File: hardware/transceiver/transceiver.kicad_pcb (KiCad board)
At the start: 4 copper layers, 30 x 30 mm, 49 parts, among them J1 Conn_01x04, J2 Conn_01x02, J3 Conn_Coaxial, U1 SX1262IMLTRT, U2 AP2112K-3.3, U3 PE4259, U4 STM32U585CIUx, Y1 32MHz, Y2 Q13FC13500004, Y3 X322516MLB4SI

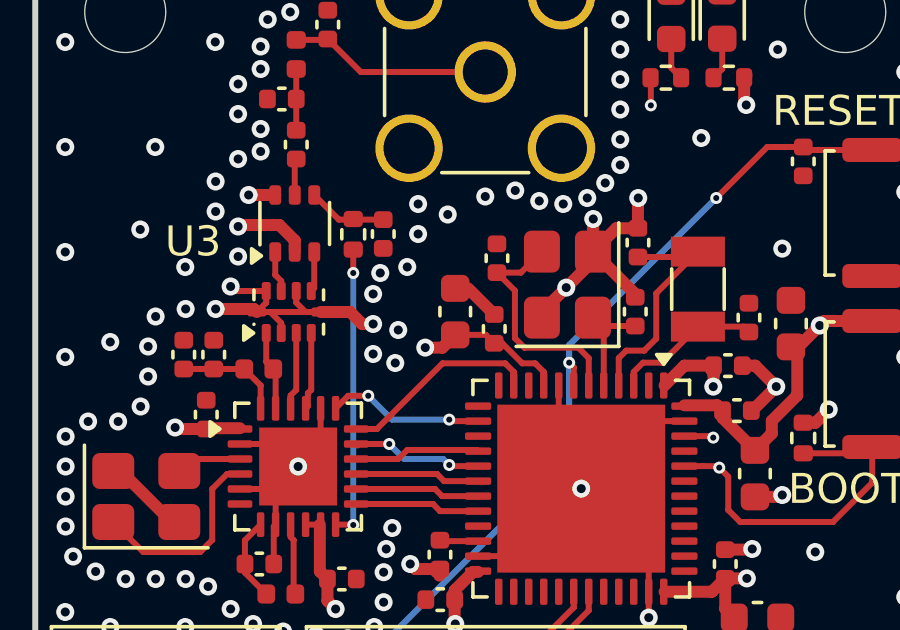
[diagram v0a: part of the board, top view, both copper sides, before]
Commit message: updated cad
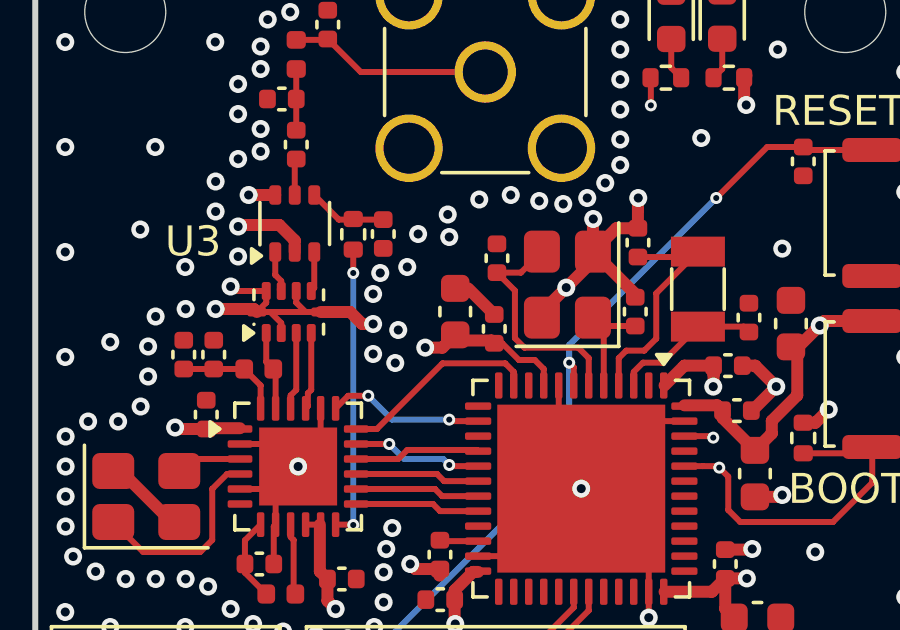
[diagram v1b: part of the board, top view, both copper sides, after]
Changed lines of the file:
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@@
 	)
 	(via
-		(at 141 102.95)
+		(at 140.85 103.1)
 		(size 0.6)
 		(drill 0.3)
@@
 	)
 	(via
-		(at 140 103.15)
+		(at 139.8 103.25)
 		(size 0.6)
 		(drill 0.3)
@@
 	)
 	(via
-		(at 137.7625 103.4)
+		(at 138.8 104.5)
 		(size 0.6)
 		(drill 0.3)
@@
 	)
 	(segment
-		(start 140.02 107.7625)
-		(end 140.3 108.0425)
+		(start 141.123703 108.6)
+		(end 141.65 108.6)
 		(width 0.2)
 		(layer "F.Cu")
@@
 	)
 	(segment
-		(start 141.664799 108.7115)
-		(end 141.95 108.996701)
-		(width 0.2)
-		(layer "F.Cu")
-		(net 3)
-	)
-	(segment
 		(start 148 115.88)
 		(end 147.555 116.325)
@@
 	)
 	(segment
-		(start 141.235203 108.7115)
-		(end 141.664799 108.7115)
+		(start 141.65 108.6)
+		(end 141.95 108.9)
+		(width 0.2)
+		(layer "F.Cu")
+		(net 3)
+	)
+	(segment
+		(start 140.3 108.0425)
+		(end 140.566203 108.0425)
 		(width 0.2)
 		(layer "F.Cu")
@@
 	)
 	(segment
-		(start 141.95 108.996701)
-		(end 141.95 109.45)
-		(width 0.2)
-		(layer "F.Cu")
-		(net 3)
-	)
-	(segment
 		(start 129.7125 110.9)
 		(end 130.7 110.9)
@@
 	)
 	(segment
-		(start 140.566203 108.0425)
-		(end 141.235203 108.7115)
-		(width 0.2)
+		(start 140.2075 107.95)
+		(end 140.3 108.0425)
+		(width 0.4)
 		(layer "F.Cu")
 		(net 3)
@@
 	)
 	(segment
-		(start 139 107.7625)
-		(end 140.02 107.7625)
-		(width 0.2)
-		(layer "F.Cu")
-		(net 3)
-	)
-	(segment
 		(start 147.555 116.325)
 		(end 145.976 116.325)
@@
 	)
 	(segment
-		(start 139.28 108.0425)
-		(end 139 107.7625)
-		(width 0.2)
-		(layer "F.Cu")
-		(net 3)
-	)
-	(segment
 		(start 147.609949 108.7875)
 		(end 146.6385 108.7875)
@@
 	)
 	(segment
+		(start 141.95 108.9)
+		(end 141.95 109.45)
+		(width 0.2)
+		(layer "F.Cu")
+		(net 3)
+	)
+	(segment
 		(start 147.909949 110.2875)
 		(end 147.909949 110.5325)
@@
 	)
 	(segment
+		(start 139.1875 107.95)
+		(end 140.2075 107.95)
+		(width 0.4)
+		(layer "F.Cu")
+		(net 3)
+	)
+	(segment
 		(start 134.74 115.9)
 		(end 134.4865 115.6465)
@@
 	)
 	(segment
-		(start 140.3 108.0425)
-		(end 140.566203 108.0425)
-		(width 0.2)
-		(layer "F.Cu")
-		(net 3)
-	)
-	(segment
 		(start 138.575 108.1875)
 		(end 139 107.7625)
@@
 	)
 	(segment
+		(start 140.566203 108.0425)
+		(end 141.123703 108.6)
+		(width 0.2)
+		(layer "F.Cu")
+		(net 3)
+	)
+	(segment
 		(start 138.98 116.5875)
 		(end 138.98 117.38)
@@
 		(start 147.909949 110.2875)
 		(end 147.733949 110.1115)
+		(width 0.4)
+		(layer "F.Cu")
+		(net 3)
+	)
+	(segment
+		(start 139 107.7625)
+		(end 139.1875 107.95)
 		(width 0.4)
 		(layer "F.Cu")
@@
 		(width 0.2)
 		(layer "F.Cu")
-		(net 22)
-	)
-	(segment
-		(start 135.749999 111.449999)
-		(end 135.7 111.4)
-		(width 0.2)
-		(layer "F.Cu")
